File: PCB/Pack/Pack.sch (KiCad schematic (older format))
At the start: 1 part

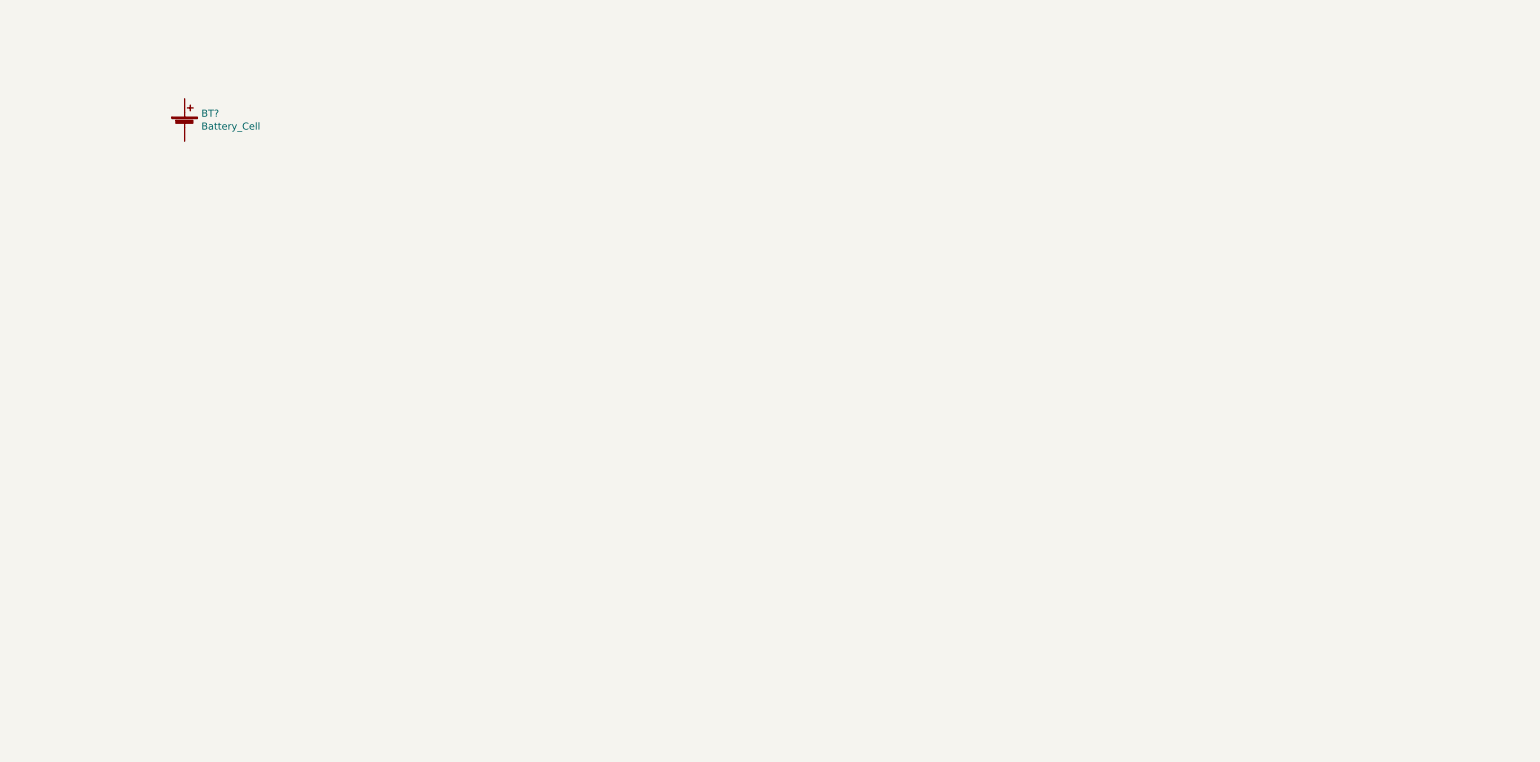
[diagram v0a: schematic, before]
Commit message: pack schematic & pcb
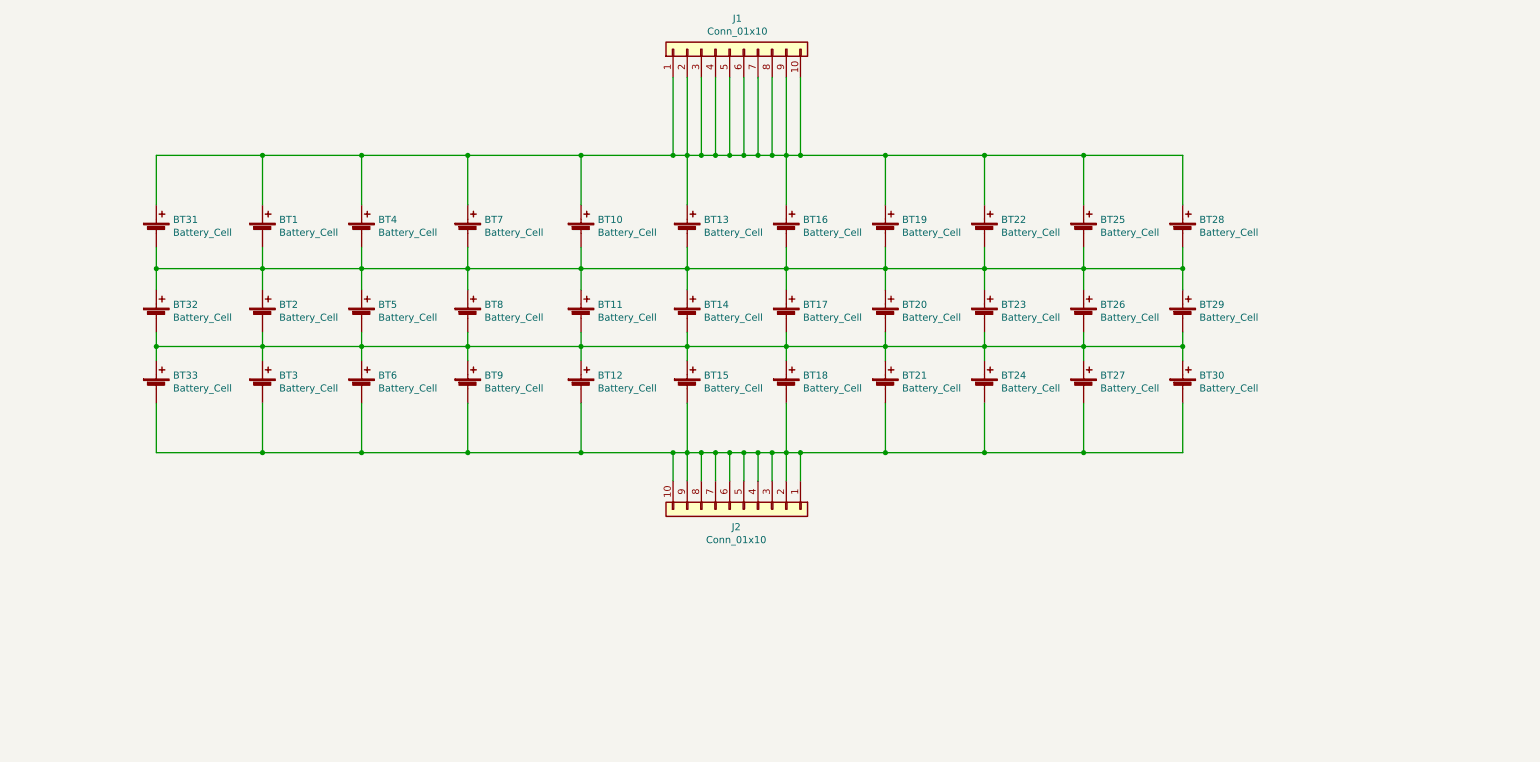
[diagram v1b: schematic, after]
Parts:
- removed BT?: Battery_Cell, symbol Device:Battery_Cell
- added BT1, BT10, BT11, BT12, BT13, BT14, BT15, BT16, BT17, BT18, BT19, BT2, BT20, BT21, BT22, BT23, BT24, BT25, BT26, BT27, BT28, BT29, BT3, BT30, BT31, BT32, BT33, BT4, BT5, BT6, BT7, BT8, BT9: Battery_Cell, ENNOID:Battery, symbol Device:Battery_Cell
- added J1, J2: Conn_01x10, symbol Connector_Generic:Conn_01x10
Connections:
- new net: BT1.1 (+), BT10.1 (+), BT13.1 (+), BT16.1 (+), BT19.1 (+), BT22.1 (+), BT25.1 (+), BT28.1 (+), BT31.1 (+), BT4.1 (+), BT7.1 (+), J1.1 (Pin_1), J1.10 (Pin_10), J1.2 (Pin_2), J1.3 (Pin_3), J1.4 (Pin_4), J1.5 (Pin_5), J1.6 (Pin_6), J1.7 (Pin_7), J1.8 (Pin_8), J1.9 (Pin_9)
- new net: BT1.2 (-), BT10.2 (-), BT11.1 (+), BT13.2 (-), BT14.1 (+), BT16.2 (-), BT17.1 (+), BT19.2 (-), BT2.1 (+), BT20.1 (+), BT22.2 (-), BT23.1 (+), BT25.2 (-), BT26.1 (+), BT28.2 (-), BT29.1 (+), BT31.2 (-), BT32.1 (+), BT4.2 (-), BT5.1 (+), BT7.2 (-), BT8.1 (+)
- new net: BT11.2 (-), BT12.1 (+), BT14.2 (-), BT15.1 (+), BT17.2 (-), BT18.1 (+), BT2.2 (-), BT20.2 (-), BT21.1 (+), BT23.2 (-), BT24.1 (+), BT26.2 (-), BT27.1 (+), BT29.2 (-), BT3.1 (+), BT30.1 (+), BT32.2 (-), BT33.1 (+), BT5.2 (-), BT6.1 (+), BT8.2 (-), BT9.1 (+)
- new net: BT12.2 (-), BT15.2 (-), BT18.2 (-), BT21.2 (-), BT24.2 (-), BT27.2 (-), BT3.2 (-), BT30.2 (-), BT33.2 (-), BT6.2 (-), BT9.2 (-), J2.1 (Pin_1), J2.10 (Pin_10), J2.2 (Pin_2), J2.3 (Pin_3), J2.4 (Pin_4), J2.5 (Pin_5), J2.6 (Pin_6), J2.7 (Pin_7), J2.8 (Pin_8), J2.9 (Pin_9)

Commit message: pack update
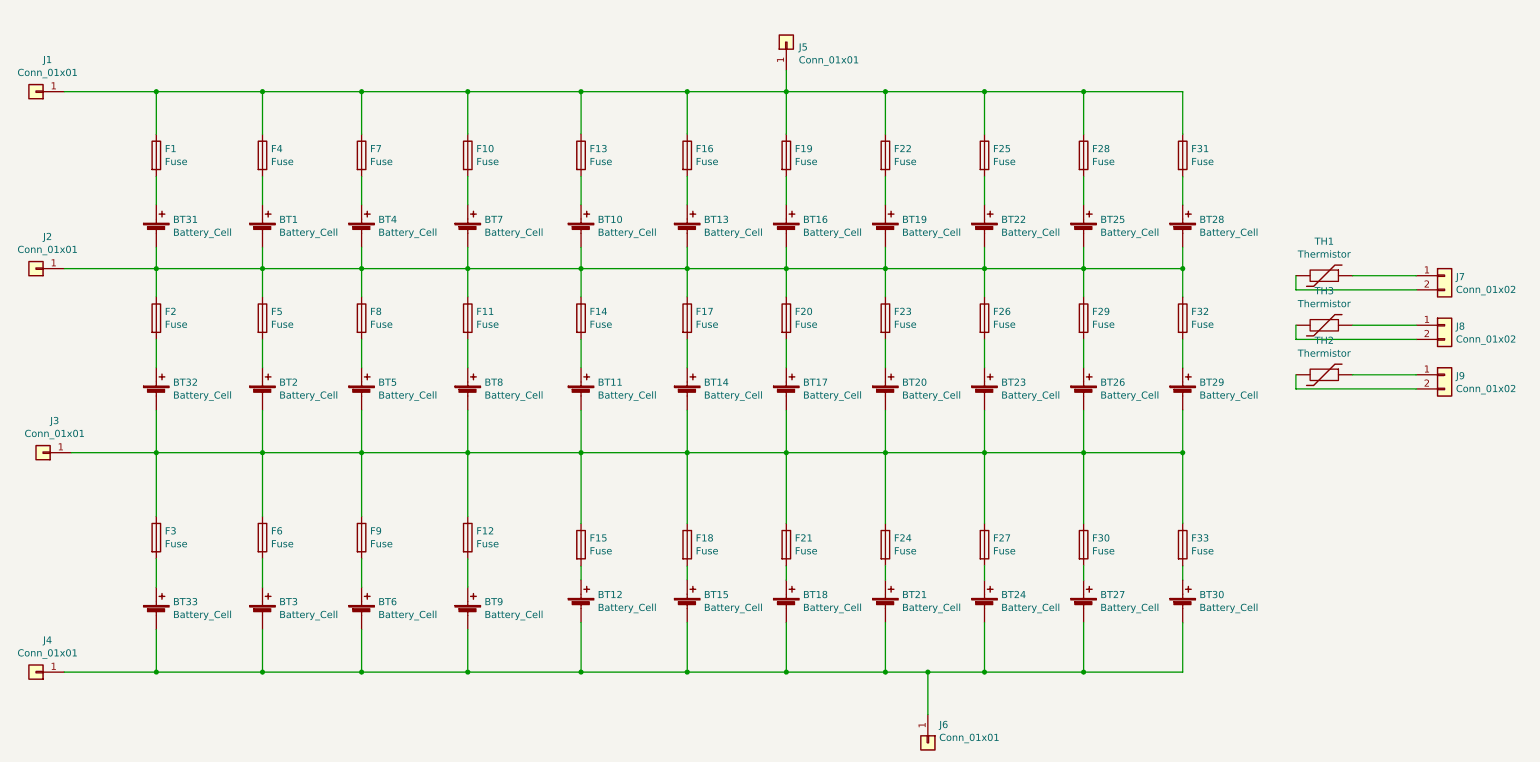
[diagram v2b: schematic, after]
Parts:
- removed J1, J2: Conn_01x10, symbol Connector_Generic:Conn_01x10
- added F1, F10, F11, F12, F13, F14, F15, F16, F17, F18, F19, F2, F20, F21, F22, F23, F24, F25, F26, F27, F28, F29, F3, F30, F31, F32, F33, F4, F5, F6, F7, F8, F9: Fuse, Resistors_SMD:R_0805, symbol Device:Fuse
- added J1, J2, J3, J4: Conn_01x01, Pin_Headers:Pin_Header_Straight_1x01_Pitch2.54mm, symbol Connector_Generic:Conn_01x01
- added J5, J6: Conn_01x01, ENNOID:Pack, symbol Connector_Generic:Conn_01x01
- added J7, J8, J9: Conn_01x02, Pin_Headers:Pin_Header_Straight_1x02_Pitch2.54mm, symbol Connector_Generic:Conn_01x02
- added TH1, TH2, TH3: Thermistor, Resistors_THT:R_Axial_DIN0309_L9.0mm_D3.2mm_P5.08mm_Vertical, symbol Device:Thermistor
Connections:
- net at BT1.2 (-), BT10.2 (-), BT13.2 (-)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: now also F11.1, F14.1, F17.1, F2.1, F20.1, F23.1, F26.1, F29.1, F32.1, F5.1, F8.1, J2.1 (Pin_1); no longer BT11.1 (+), BT14.1 (+), BT17.1 (+), BT2.1 (+), BT20.1 (+), BT23.1 (+), BT26.1 (+), BT29.1 (+), BT32.1 (+), BT5.1 (+), BT8.1 (+)
- net at BT11.2 (-), BT14.2 (-), BT17.2 (-)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: now also F12.1, F15.1, F18.1, F21.1, F24.1, F27.1, F3.1, F30.1, F33.1, F6.1, F9.1, J3.1 (Pin_1); no longer BT12.1 (+), BT15.1 (+), BT18.1 (+), BT21.1 (+), BT24.1 (+), BT27.1 (+), BT3.1 (+), BT30.1 (+), BT33.1 (+), BT6.1 (+), BT9.1 (+)
- net at BT12.2 (-), BT15.2 (-), BT18.2 (-)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: now also J4.1 (Pin_1), J6.1 (Pin_1)
- new net: BT1.1 (+), F4.2
- new net: BT4.1 (+), F7.2
- new net: BT7.1 (+), F10.2
- new net: BT10.1 (+), F13.2
- new net: BT13.1 (+), F16.2
- new net: BT16.1 (+), F19.2
- new net: BT19.1 (+), F22.2
- new net: BT22.1 (+), F25.2
- new net: BT25.1 (+), F28.2
- new net: BT28.1 (+), F31.2
- new net: BT2.1 (+), F5.2
- new net: BT5.1 (+), F8.2
- new net: BT8.1 (+), F11.2
- new net: BT11.1 (+), F14.2
- new net: BT14.1 (+), F17.2
- new net: BT17.1 (+), F20.2
- new net: BT20.1 (+), F23.2
- new net: BT23.1 (+), F26.2
- new net: BT26.1 (+), F29.2
- new net: BT29.1 (+), F32.2
- new net: BT3.1 (+), F6.2
- new net: BT6.1 (+), F9.2
- new net: BT9.1 (+), F12.2
- new net: BT12.1 (+), F15.2
- new net: BT15.1 (+), F18.2
- new net: BT18.1 (+), F21.2
- new net: BT21.1 (+), F24.2
- new net: BT24.1 (+), F27.2
- new net: BT27.1 (+), F30.2
- new net: BT30.1 (+), F33.2
- new net: BT31.1 (+), F1.2
- new net: BT32.1 (+), F2.2
- new net: BT33.1 (+), F3.2
- new net: J7.1 (Pin_1), TH1.1
- new net: J7.2 (Pin_2), TH1.2
- new net: F1.1, F10.1, F13.1, F16.1, F19.1, F22.1, F25.1, F28.1, F31.1, F4.1, F7.1, J1.1 (Pin_1), J5.1 (Pin_1)
- new net: J9.1 (Pin_1), TH2.1
- new net: J9.2 (Pin_2), TH2.2
- new net: J8.1 (Pin_1), TH3.1
- new net: J8.2 (Pin_2), TH3.2
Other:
- moved on the sheet: BT11, BT12, BT14, BT15, BT17, BT18, BT2, BT20, BT21, BT23, BT24, BT26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

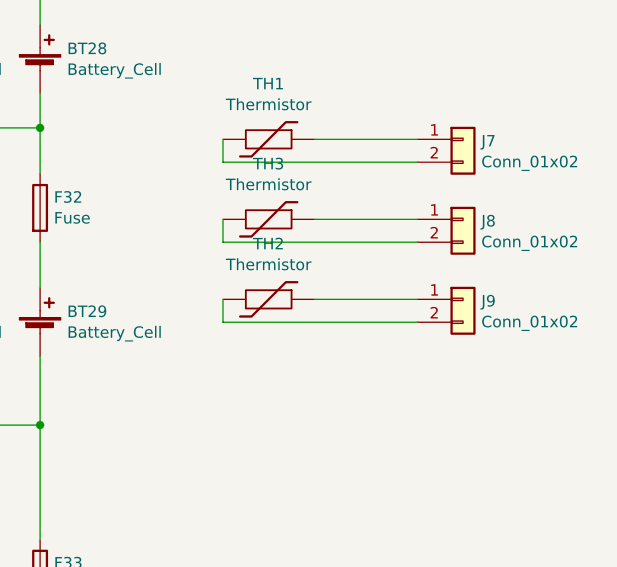
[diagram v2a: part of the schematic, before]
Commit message: Pack completed
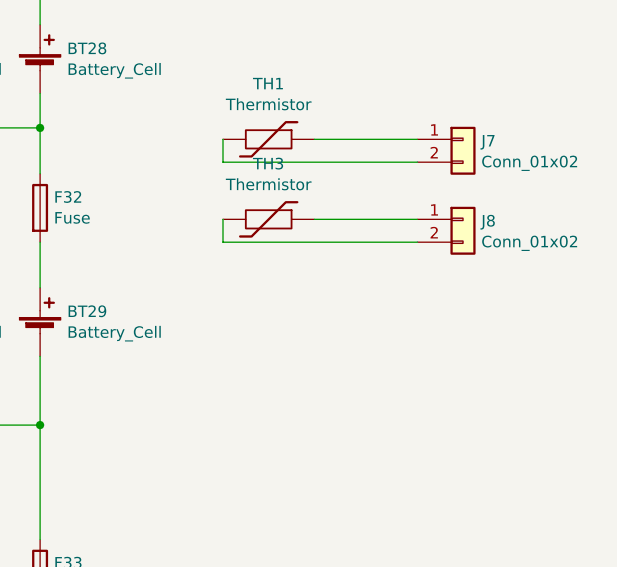
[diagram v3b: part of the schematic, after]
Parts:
- removed J9: Conn_01x02, Pin_Headers:Pin_Header_Straight_1x02_Pitch2.54mm, symbol Connector_Generic:Conn_01x02
- removed TH2: Thermistor, Resistors_THT:R_Axial_DIN0309_L9.0mm_D3.2mm_P5.08mm_Vertical, symbol Device:Thermistor
- F1, F10, F11, F12, F13, F14, F15, F16, F17, F18, F19, F2, F20, F21, F22, F23, F24, F25, F26, F27, F28, F29, F3, F30, F31, F32, F33, F4, F5, F6, F7, F8, F9: footprint Resistors_SMD:R_0805 -> Fuse_Holders_and_Fuses:Fuse_SMD1206_Wave
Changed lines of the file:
@@
-	0    1    1    0
-$EndComp
-$Comp
-L Device:Thermistor TH2
-U 1 1 5C69E246
-P 9800 3300
-F 0 "TH2" V 9558 3300 50  0000 C CNN
-F 1 "Thermistor" V 9649 3300 50  0000 C CNN
-F 2 "Resistors_THT:R_Axial_DIN0309_L9.0mm_D3.2mm_P5.08mm_Vertical" H 9800 3300 50  0001 C CNN
-F 3 "~" H 9800 3300 50  0001 C CNN
-	1    9800 3300
 	0    1    1    0
 $EndComp
@@
 	10000 2600 10450 2600
 Wire Wire Line
-	10000 3300 10450 3300
-Wire Wire Line
 	7000 5400 7400 5400
 $Comp
@@
 	1    0    0    -1
 $EndComp
-$Comp
-L Connector_Generic:Conn_01x02 J9
-U 1 1 5C99C270
-P 10650 3300
-F 0 "J9" H 10730 3292 50  0000 L CNN
-F 1 "Conn_01x02" H 10730 3201 50  0000 L CNN
-F 2 "Pin_Headers:Pin_Header_Straight_1x02_Pitch2.54mm" H 10650 3300 50  0001 C CNN
-F 3 "~" H 10650 3300 50  0001 C CNN
-	1    10650 3300
-	1    0    0    -1
-$EndComp
 Wire Wire Line
 	10450 2700 9600 2700
@@
 Wire Wire Line
 	9600 3050 9600 2950
-Wire Wire Line
-	10450 3400 9600 3400
-Wire Wire Line
-	9600 3400 9600 3300
 Wire Wire Line
 	8800 5400 8800 5050
@@
 F 0 "F3" H 1610 4496 50  0000 L CNN
 F 1 "Fuse" H 1610 4405 50  0000 L CNN
-F 2 "Resistors_SMD:R_0805" V 1480 4450 50  0001 C CNN
+F 2 "Fuse_Holders_and_Fuses:Fuse_SMD1206_Wave" V 1480 4450 50  0001 C CNN
 F 3 "~" H 1550 4450 50  0001 C CNN
 	1    1550 4450
@@
 F 0 "F6" H 2360 4496 50  0000 L CNN
 F 1 "Fuse" H 2360 4405 50  0000 L CNN
-F 2 "Resistors_SMD:R_0805" V 2230 4450 50  0001 C CNN
+F 2 "Fuse_Holders_and_Fuses:Fuse_SMD1206_Wave" V 2230 4450 50  0001 C CNN
 F 3 "~" H 2300 4450 50  0001 C CNN
 	1    2300 4450
@@
 F 0 "F9" H 3060 4496 50  0000 L CNN
 F 1 "Fuse" H 3060 4405 50  0000 L CNN
-F 2 "Resistors_SMD:R_0805" V 2930 4450 50  0001 C CNN
+F 2 "Fuse_Holders_and_Fuses:Fuse_SMD1206_Wave" V 2930 4450 50  0001 C CNN
 F 3 "~" H 3000 4450 50  0001 C CNN
 	1    3000 4450
@@
 F 0 "F12" H 3810 4496 50  0000 L CNN
 F 1 "Fuse" H 3810 4405 50  0000 L CNN
-F 2 "Resistors_SMD:R_0805" V 3680 4450 50  0001 C CNN
+F 2 "Fuse_Holders_and_Fuses:Fuse_SMD1206_Wave" V 3680 4450 50  0001 C CNN
 F 3 "~" H 3750 4450 50  0001 C CNN
 	1    3750 4450
@@
 F 0 "F15" H 4610 4546 50  0000 L CNN
 F 1 "Fuse" H 4610 4455 50  0000 L CNN
-F 2 "Resistors_SMD:R_0805" V 4480 4500 50  0001 C CNN
+F 2 "Fuse_Holders_and_Fuses:Fuse_SMD1206_Wave" V 4480 4500 50  0001 C CNN
 F 3 "~" H 4550 4500 50  0001 C CNN
 	1    4550 4500
@@
 F 0 "F18" H 5360 4546 50  0000 L CNN
 F 1 "Fuse" H 5360 4455 50  0000 L CNN
-F 2 "Resistors_SMD:R_0805" V 5230 4500 50  0001 C CNN
+F 2 "Fuse_Holders_and_Fuses:Fuse_SMD1206_Wave" V 5230 4500 50  0001 C CNN
 F 3 "~" H 5300 4500 50  0001 C CNN
 	1    5300 4500
@@
 F 0 "F21" H 6060 4546 50  0000 L CNN
 F 1 "Fuse" H 6060 4455 50  0000 L CNN
-F 2 "Resistors_SMD:R_0805" V 5930 4500 50  0001 C CNN
+F 2 "Fuse_Holders_and_Fuses:Fuse_SMD1206_Wave" V 5930 4500 50  0001 C CNN
 F 3 "~" H 6000 4500 50  0001 C CNN
 	1    6000 4500
@@
 F 0 "F24" H 6760 4546 50  0000 L CNN
 F 1 "Fuse" H 6760 4455 50  0000 L CNN
-F 2 "Resistors_SMD:R_0805" V 6630 4500 50  0001 C CNN
+F 2 "Fuse_Holders_and_Fuses:Fuse_SMD1206_Wave" V 6630 4500 50  0001 C CNN
 F 3 "~" H 6700 4500 50  0001 C CNN
 	1    6700 4500
@@
 F 0 "F27" H 7460 4546 50  0000 L CNN
 F 1 "Fuse" H 7460 4455 50  0000 L CNN
-F 2 "Resistors_SMD:R_0805" V 7330 4500 50  0001 C CNN
+F 2 "Fuse_Holders_and_Fuses:Fuse_SMD1206_Wave" V 7330 4500 50  0001 C CNN
 F 3 "~" H 7400 4500 50  0001 C CNN
 	1    7400 4500
@@
 F 0 "F30" H 8160 4546 50  0000 L CNN
 F 1 "Fuse" H 8160 4455 50  0000 L CNN
-F 2 "Resistors_SMD:R_0805" V 8030 4500 50  0001 C CNN
+F 2 "Fuse_Holders_and_Fuses:Fuse_SMD1206_Wave" V 8030 4500 50  0001 C CNN
 F 3 "~" H 8100 4500 50  0001 C CNN
 	1    8100 4500
@@
 F 0 "F33" H 8860 4546 50  0000 L CNN
 F 1 "Fuse" H 8860 4455 50  0000 L CNN
-F 2 "Resistors_SMD:R_0805" V 8730 4500 50  0001 C CNN
+F 2 "Fuse_Holders_and_Fuses:Fuse_SMD1206_Wave" V 8730 4500 50  0001 C CNN
 F 3 "~" H 8800 4500 50  0001 C CNN
 	1    8800 4500
@@
 F 0 "F2" H 1610 2946 50  0000 L CNN
 F 1 "Fuse" H 1610 2855 50  0000 L CNN
-F 2 "Resistors_SMD:R_0805" V 1480 2900 50  0001 C CNN
+F 2 "Fuse_Holders_and_Fuses:Fuse_SMD1206_Wave" V 1480 2900 50  0001 C CNN
 F 3 "~" H 1550 2900 50  0001 C CNN
 	1    1550 2900
@@
 F 0 "F5" H 2360 2946 50  0000 L CNN
 F 1 "Fuse" H 2360 2855 50  0000 L CNN
-F 2 "Resistors_SMD:R_0805" V 2230 2900 50  0001 C CNN
+F 2 "Fuse_Holders_and_Fuses:Fuse_SMD1206_Wave" V 2230 2900 50  0001 C CNN
 F 3 "~" H 2300 2900 50  0001 C CNN
 	1    2300 2900
@@
 F 0 "F8" H 3060 2946 50  0000 L CNN
 F 1 "Fuse" H 3060 2855 50  0000 L CNN
-F 2 "Resistors_SMD:R_0805" V 2930 2900 50  0001 C CNN
+F 2 "Fuse_Holders_and_Fuses:Fuse_SMD1206_Wave" V 2930 2900 50  0001 C CNN
 F 3 "~" H 3000 2900 50  0001 C CNN
 	1    3000 2900
@@
 F 0 "F11" H 3810 2946 50  0000 L CNN
 F 1 "Fuse" H 3810 2855 50  0000 L CNN
-F 2 "Resistors_SMD:R_0805" V 3680 2900 50  0001 C CNN
+F 2 "Fuse_Holders_and_Fuses:Fuse_SMD1206_Wave" V 3680 2900 50  0001 C CNN
 F 3 "~" H 3750 2900 50  0001 C CNN
 	1    3750 2900
@@
 F 0 "F14" H 4610 2946 50  0000 L CNN
 F 1 "Fuse" H 4610 2855 50  0000 L CNN
-F 2 "Resistors_SMD:R_0805" V 4480 2900 50  0001 C CNN
+F 2 "Fuse_Holders_and_Fuses:Fuse_SMD1206_Wave" V 4480 2900 50  0001 C CNN
 F 3 "~" H 4550 2900 50  0001 C CNN
 	1    4550 2900
@@
 F 0 "F17" H 5360 2946 50  0000 L CNN
 F 1 "Fuse" H 5360 2855 50  0000 L CNN
-F 2 "Resistors_SMD:R_0805" V 5230 2900 50  0001 C CNN
+F 2 "Fuse_Holders_and_Fuses:Fuse_SMD1206_Wave" V 5230 2900 50  0001 C CNN
 F 3 "~" H 5300 2900 50  0001 C CNN
 	1    5300 2900
@@
 F 0 "F20" H 6060 2946 50  0000 L CNN
 F 1 "Fuse" H 6060 2855 50  0000 L CNN
-F 2 "Resistors_SMD:R_0805" V 5930 2900 50  0001 C CNN
+F 2 "Fuse_Holders_and_Fuses:Fuse_SMD1206_Wave" V 5930 2900 50  0001 C CNN
 F 3 "~" H 6000 2900 50  0001 C CNN
 	1    6000 2900
@@
 F 0 "F23" H 6760 2946 50  0000 L CNN
 F 1 "Fuse" H 6760 2855 50  0000 L CNN
-F 2 "Resistors_SMD:R_0805" V 6630 2900 50  0001 C CNN
+F 2 "Fuse_Holders_and_Fuses:Fuse_SMD1206_Wave" V 6630 2900 50  0001 C CNN
 F 3 "~" H 6700 2900 50  0001 C CNN
 	1    6700 2900
@@
 F 0 "F26" H 7460 2946 50  0000 L CNN
 F 1 "Fuse" H 7460 2855 50  0000 L CNN
-F 2 "Resistors_SMD:R_0805" V 7330 2900 50  0001 C CNN
+F 2 "Fuse_Holders_and_Fuses:Fuse_SMD1206_Wave" V 7330 2900 50  0001 C CNN
 F 3 "~" H 7400 2900 50  0001 C CNN
 	1    7400 2900
@@
 F 0 "F29" H 8160 2946 50  0000 L CNN
 F 1 "Fuse" H 8160 2855 50  0000 L CNN
-F 2 "Resistors_SMD:R_0805" V 8030 2900 50  0001 C CNN
+F 2 "Fuse_Holders_and_Fuses:Fuse_SMD1206_Wave" V 8030 2900 50  0001 C CNN
 F 3 "~" H 8100 2900 50  0001 C CNN
 	1    8100 2900
@@
 F 0 "F32" H 8860 2946 50  0000 L CNN
 F 1 "Fuse" H 8860 2855 50  0000 L CNN
-F 2 "Resistors_SMD:R_0805" V 8730 2900 50  0001 C CNN
+F 2 "Fuse_Holders_and_Fuses:Fuse_SMD1206_Wave" V 8730 2900 50  0001 C CNN
 F 3 "~" H 8800 2900 50  0001 C CNN
 	1    8800 2900
@@
 F 0 "F31" H 8860 1796 50  0000 L CNN
 F 1 "Fuse" H 8860 1705 50  0000 L CNN
-F 2 "Resistors_SMD:R_0805" V 8730 1750 50  0001 C CNN
+F 2 "Fuse_Holders_and_Fuses:Fuse_SMD1206_Wave" V 8730 1750 50  0001 C CNN
 F 3 "~" H 8800 1750 50  0001 C CNN
 	1    8800 1750
@@
 F 0 "F28" H 8160 1796 50  0000 L CNN
 F 1 "Fuse" H 8160 1705 50  0000 L CNN
-F 2 "Resistors_SMD:R_0805" V 8030 1750 50  0001 C CNN
+F 2 "Fuse_Holders_and_Fuses:Fuse_SMD1206_Wave" V 8030 1750 50  0001 C CNN
 F 3 "~" H 8100 1750 50  0001 C CNN
 	1    8100 1750
@@
 F 0 "F25" H 7460 1796 50  0000 L CNN
 F 1 "Fuse" H 7460 1705 50  0000 L CNN
-F 2 "Resistors_SMD:R_0805" V 7330 1750 50  0001 C CNN
+F 2 "Fuse_Holders_and_Fuses:Fuse_SMD1206_Wave" V 7330 1750 50  0001 C CNN
 F 3 "~" H 7400 1750 50  0001 C CNN
 	1    7400 1750
@@
 F 0 "F22" H 6760 1796 50  0000 L CNN
 F 1 "Fuse" H 6760 1705 50  0000 L CNN
-F 2 "Resistors_SMD:R_0805" V 6630 1750 50  0001 C CNN
+F 2 "Fuse_Holders_and_Fuses:Fuse_SMD1206_Wave" V 6630 1750 50  0001 C CNN
 F 3 "~" H 6700 1750 50  0001 C CNN
 	1    6700 1750
@@
 F 0 "F19" H 6060 1796 50  0000 L CNN
 F 1 "Fuse" H 6060 1705 50  0000 L CNN
-F 2 "Resistors_SMD:R_0805" V 5930 1750 50  0001 C CNN
+F 2 "Fuse_Holders_and_Fuses:Fuse_SMD1206_Wave" V 5930 1750 50  0001 C CNN
 F 3 "~" H 6000 1750 50  0001 C CNN
 	1    6000 1750
@@
 F 0 "F16" H 5360 1796 50  0000 L CNN
 F 1 "Fuse" H 5360 1705 50  0000 L CNN
-F 2 "Resistors_SMD:R_0805" V 5230 1750 50  0001 C CNN
+F 2 "Fuse_Holders_and_Fuses:Fuse_SMD1206_Wave" V 5230 1750 50  0001 C CNN
 F 3 "~" H 5300 1750 50  0001 C CNN
 	1    5300 1750
@@
 F 0 "F13" H 4610 1796 50  0000 L CNN
 F 1 "Fuse" H 4610 1705 50  0000 L CNN
-F 2 "Resistors_SMD:R_0805" V 4480 1750 50  0001 C CNN
+F 2 "Fuse_Holders_and_Fuses:Fuse_SMD1206_Wave" V 4480 1750 50  0001 C CNN
 F 3 "~" H 4550 1750 50  0001 C CNN
 	1    4550 1750
@@
 F 0 "F10" H 3810 1796 50  0000 L CNN
 F 1 "Fuse" H 3810 1705 50  0000 L CNN
-F 2 "Resistors_SMD:R_0805" V 3680 1750 50  0001 C CNN
+F 2 "Fuse_Holders_and_Fuses:Fuse_SMD1206_Wave" V 3680 1750 50  0001 C CNN
 F 3 "~" H 3750 1750 50  0001 C CNN
 	1    3750 1750
@@
 F 0 "F7" H 3060 1796 50  0000 L CNN
 F 1 "Fuse" H 3060 1705 50  0000 L CNN
-F 2 "Resistors_SMD:R_0805" V 2930 1750 50  0001 C CNN
+F 2 "Fuse_Holders_and_Fuses:Fuse_SMD1206_Wave" V 2930 1750 50  0001 C CNN
 F 3 "~" H 3000 1750 50  0001 C CNN
 	1    3000 1750
@@
 F 0 "F4" H 2360 1796 50  0000 L CNN
 F 1 "Fuse" H 2360 1705 50  0000 L CNN
-F 2 "Resistors_SMD:R_0805" V 2230 1750 50  0001 C CNN
+F 2 "Fuse_Holders_and_Fuses:Fuse_SMD1206_Wave" V 2230 1750 50  0001 C CNN
 F 3 "~" H 2300 1750 50  0001 C CNN
 	1    2300 1750
@@
 F 0 "F1" H 1610 1796 50  0000 L CNN
 F 1 "Fuse" H 1610 1705 50  0000 L CNN
-F 2 "Resistors_SMD:R_0805" V 1480 1750 50  0001 C CNN
+F 2 "Fuse_Holders_and_Fuses:Fuse_SMD1206_Wave" V 1480 1750 50  0001 C CNN
 F 3 "~" H 1550 1750 50  0001 C CNN
 	1    1550 1750
